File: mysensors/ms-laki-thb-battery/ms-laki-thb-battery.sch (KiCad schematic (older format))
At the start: 2 parts, among them U1 MCP1640CH

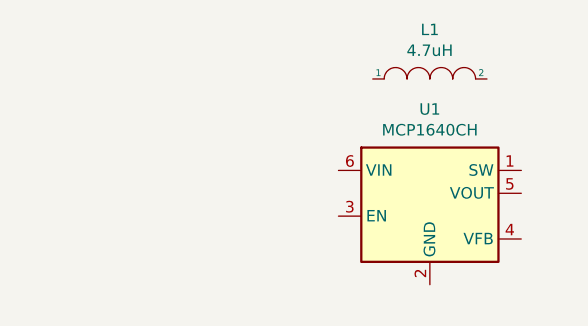
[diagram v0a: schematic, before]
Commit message: .
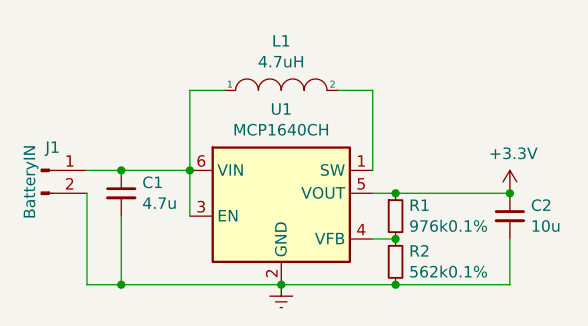
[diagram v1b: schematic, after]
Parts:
- added C1: 4.7u, Capacitor_SMD:C_1206_3216Metric_Pad1.42x1.75mm_HandSolder, symbol Device:C_Small
- added C2: 10u, Capacitor_SMD:C_1206_3216Metric_Pad1.42x1.75mm_HandSolder, symbol Device:C_Small
- added J1: BatteryIN, Connector_PinHeader_2.54mm:PinHeader_1x02_P2.54mm_Vertical, symbol Connector:Conn_01x02_Male
- added R1: 976k0.1%, Resistor_THT:R_Axial_DIN0207_L6.3mm_D2.5mm_P7.62mm_Horizontal, symbol Device:R_Small
- added R2: 562k0.1%, Resistor_THT:R_Axial_DIN0207_L6.3mm_D2.5mm_P7.62mm_Horizontal, symbol Device:R_Small
- L1: footprint (none) -> Inductor_SMD:L_Taiyo-Yuden_NR-60xx_HandSoldering; PN (none) -> 1003.7128; Price[HUF] (none) -> 27.3; Supplier (none) -> hestore
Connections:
- net at U1.1 (SW): now also L1.2
- net Earth: now reaches U1.2 (GND)
- net Earth: now also C1.2, C2.2, J1.2 (Pin_2), R2.2
- net at U1.3 (EN): now also L1.1, U1.6 (VIN), C1.1, J1.1 (Pin_1)
- net at U1.4 (VFB): now also R1.2, R2.1
- net +3V3: now reaches U1.5 (VOUT)
- net +3V3: now also C2.1, R1.1
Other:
- moved on the sheet: L1, U1
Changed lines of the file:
@@
 EESchema Schematic File Version 4
+LIBS:ms-laki-thb-battery-cache
 EELAYER 26 0
 EELAYER END
@@
 L Regulator_Switching:MCP1640CH U1
 U 1 1 5C2F1D67
-P 2350 1500
-F 0 "U1" H 2350 1967 50  0000 C CNN
-F 1 "MCP1640CH" H 2350 1876 50  0000 C CNN
-F 2 "Package_TO_SOT_SMD:SOT-23-6" H 2400 1250 50  0001 L CIN
-F 3 "http://ww1.microchip.com/downloads/en/DeviceDoc/20002234D.pdf" H 2100 1950 50  0001 C CNN
-F 4 "hestore" H 2350 1500 50  0001 C CNN "Supplier"
-F 5 "1003.2042" H 2350 1500 50  0001 C CNN "PN"
-F 6 "227" H 2350 1500 50  0001 C CNN "Price[HUF]"
-	1    2350 1500
+P 1700 1500
+F 0 "U1" H 1700 1967 50  0000 C CNN
+F 1 "MCP1640CH" H 1700 1876 50  0000 C CNN
+F 2 "Package_TO_SOT_SMD:SOT-23-6" H 1750 1250 50  0001 L CIN
+F 3 "http://ww1.microchip.com/downloads/en/DeviceDoc/20002234D.pdf" H 1450 1950 50  0001 C CNN
+F 4 "hestore" H 1700 1500 50  0001 C CNN "Supplier"
+F 5 "1003.2042" H 1700 1500 50  0001 C CNN "PN"
+F 6 "227" H 1700 1500 50  0001 C CNN "Price[HUF]"
+	1    1700 1500
 	1    0    0    -1
 $EndComp
@@
 L pspice:INDUCTOR L1
 U 1 1 5C2F1ED2
-P 2350 900
-F 0 "L1" H 2350 1115 50  0000 C CNN
-F 1 "4.7uH" H 2350 1024 50  0000 C CNN
-F 2 "" H 2350 900 50  0001 C CNN
-F 3 "~" H 2350 900 50  0001 C CNN
-	1    2350 900
+P 1700 950
+F 0 "L1" H 1700 1165 50  0000 C CNN
+F 1 "4.7uH" H 1700 1074 50  0000 C CNN
+F 2 "Inductor_SMD:L_Taiyo-Yuden_NR-60xx_HandSoldering" H 1700 950 50  0001 C CNN
+F 3 "~" H 1700 950 50  0001 C CNN
+F 4 "hestore" H 1700 950 50  0001 C CNN "Supplier"
+F 5 "1003.7128" H 1700 950 50  0001 C CNN "PN"
+F 6 "27.3" H 1700 950 50  0001 C CNN "Price[HUF]"
+	1    1700 950
 	1    0    0    -1
 $EndComp
+$Comp
+L Device:C_Small C1
+U 1 1 5C2FBC1E
+P 1000 1400
+F 0 "C1" H 1092 1446 50  0000 L CNN
+F 1 "4.7u" H 1092 1355 50  0000 L CNN
+F 2 "Capacitor_SMD:C_1206_3216Metric_Pad1.42x1.75mm_HandSolder" H 1000 1400 50  0001 C CNN
+F 3 "https://www.hestore.hu/prod_getfile.php?id=3608" H 1000 1400 50  0001 C CNN
+F 4 "hestore" H 1000 1400 50  0001 C CNN "Supplier"
+F 5 "1000.0405" H 1000 1400 50  0001 C CNN "PN"
+F 6 "8" H 1000 1400 50  0001 C CNN "Price[HUF]"
+	1    1000 1400
+	1    0    0    -1
+$EndComp
+$Comp
+L Device:C_Small C2
+U 1 1 5C2FBCD6
+P 2700 1500
+F 0 "C2" H 2792 1546 50  0000 L CNN
+F 1 "10u" H 2792 1455 50  0000 L CNN
+F 2 "Capacitor_SMD:C_1206_3216Metric_Pad1.42x1.75mm_HandSolder" H 2700 1500 50  0001 C CNN
+F 3 "~" H 2700 1500 50  0001 C CNN
+F 4 "hestore" H 2700 1500 50  0001 C CNN "Supplier"
+F 5 "1003.1528" H 2700 1500 50  0001 C CNN "PN"
+F 6 "45.6" H 2700 1500 50  0001 C CNN "Price[HUF]"
+	1    2700 1500
+	1    0    0    -1
+$EndComp
+$Comp
+L Device:R_Small R1
+U 1 1 5C2FBDB7
+P 2200 1500
+F 0 "R1" H 2259 1546 50  0000 L CNN
+F 1 "976k0.1%" H 2259 1455 50  0000 L CNN
+F 2 "Resistor_THT:R_Axial_DIN0207_L6.3mm_D2.5mm_P7.62mm_Horizontal" H 2200 1500 50  0001 C CNN
+F 3 "https://www.hestore.hu/prod_getfile.php?id=2836" H 2200 1500 50  0001 C CNN
+F 4 "hestore" H 2200 1500 50  0001 C CNN "Supplier"
+F 5 "1002.7492" H 2200 1500 50  0001 C CNN "PN"
+F 6 "50" H 2200 1500 50  0001 C CNN "Price[HUF]"
+	1    2200 1500
+	1    0    0    -1
+$EndComp
+$Comp
+L Device:R_Small R2
+U 1 1 5C2FBE62
+P 2200 1700
+F 0 "R2" H 2259 1746 50  0000 L CNN
+F 1 "562k0.1%" H 2259 1655 50  0000 L CNN
+F 2 "Resistor_THT:R_Axial_DIN0207_L6.3mm_D2.5mm_P7.62mm_Horizontal" H 2200 1700 50  0001 C CNN
+F 3 "https://www.hestore.hu/prod_getfile.php?id=2813" H 2200 1700 50  0001 C CNN
+F 4 "hestore" H 2200 1700 50  0001 C CNN "Supplier"
+F 5 "1002.7469" H 2200 1700 50  0001 C CNN "PN"
+F 6 "51.3" H 2200 1700 50  0001 C CNN "Price[HUF]"
+	1    2200 1700
+	1    0    0    -1
+$EndComp
+Wire Wire Line
+	1450 950  1300 950
+Wire Wire Line
+	1300 950  1300 1300
+Wire Wire Line
+	1950 950  2100 950
+Wire Wire Line
+	2100 950  2100 1300
+Wire Wire Line
+	2200 1400 2100 1400
+Wire Wire Line
+	2100 1600 2200 1600
+Connection ~ 2200 1600
+Wire Wire Line
+	2200 1800 1700 1800
+Wire Wire Line
+	1300 1500 1300 1300
+Connection ~ 1300 1300
+Wire Wire Line
+	1300 1300 1000 1300
+Wire Wire Line
+	1000 1500 1000 1800
+Wire Wire Line
+	1000 1800 1700 1800
+Connection ~ 1700 1800
+Wire Wire Line
+	2700 1400 2200 1400
+Connection ~ 2200 1400
+Wire Wire Line
+	2200 1800 2700 1800
+Wire Wire Line
+	2700 1800 2700 1600
+Connection ~ 2200 1800
+$Comp
+L power:+3.3V #PWR?
+U 1 1 5C2FC53C
+P 2700 1400
+F 0 "#PWR?" H 2700 1250 50  0001 C CNN
+F 1 "+3.3V" H 2715 1573 50  0000 C CNN
+F 2 "" H 2700 1400 50  0001 C CNN
+F 3 "" H 2700 1400 50  0001 C CNN
+	1    2700 1400
+	1    0    0    -1
+$EndComp
+Connection ~ 2700 1400
+$Comp
+L power:Earth #PWR?
+U 1 1 5C2FC631
+P 1700 1800
+F 0 "#PWR?" H 1700 1550 50  0001 C CNN
+F 1 "Earth" H 1700 1650 50  0001 C CNN
+F 2 "" H 1700 1800 50  0001 C CNN
+F 3 "~" H 1700 1800 50  0001 C CNN
+	1    1700 1800
+	1    0    0    -1
+$EndComp
+$Comp
+L Connector:Conn_01x02_Male J1
+U 1 1 5C2FC689
+P 650 1300
+F 0 "J1" H 700 1400 50  0000 C CNN
+F 1 "BatteryIN" V 600 1250 50  0000 C CNN
+F 2 "Connector_PinHeader_2.54mm:PinHeader_1x02_P2.54mm_Vertical" H 650 1300 50  0001 C CNN
+F 3 "~" H 650 1300 50  0001 C CNN
+	1    650  1300
+	1    0    0    -1
+$EndComp
+Wire Wire Line
+	850  1300 1000 1300
+Connection ~ 1000 1300
+Wire Wire Line
+	850  1400 850  1800
+Wire Wire Line
+	850  1800 1000 1800
+Connection ~ 1000 1800
 $EndSCHEMATC
